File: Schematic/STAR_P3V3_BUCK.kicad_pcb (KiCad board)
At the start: 2 copper layers, 70.1 x 70 mm, 19 parts, among them J1 1017491, J2 6120XX21621_61200621621, J3 6120XX21621_61200821621, U1 TLV62569ADRLR

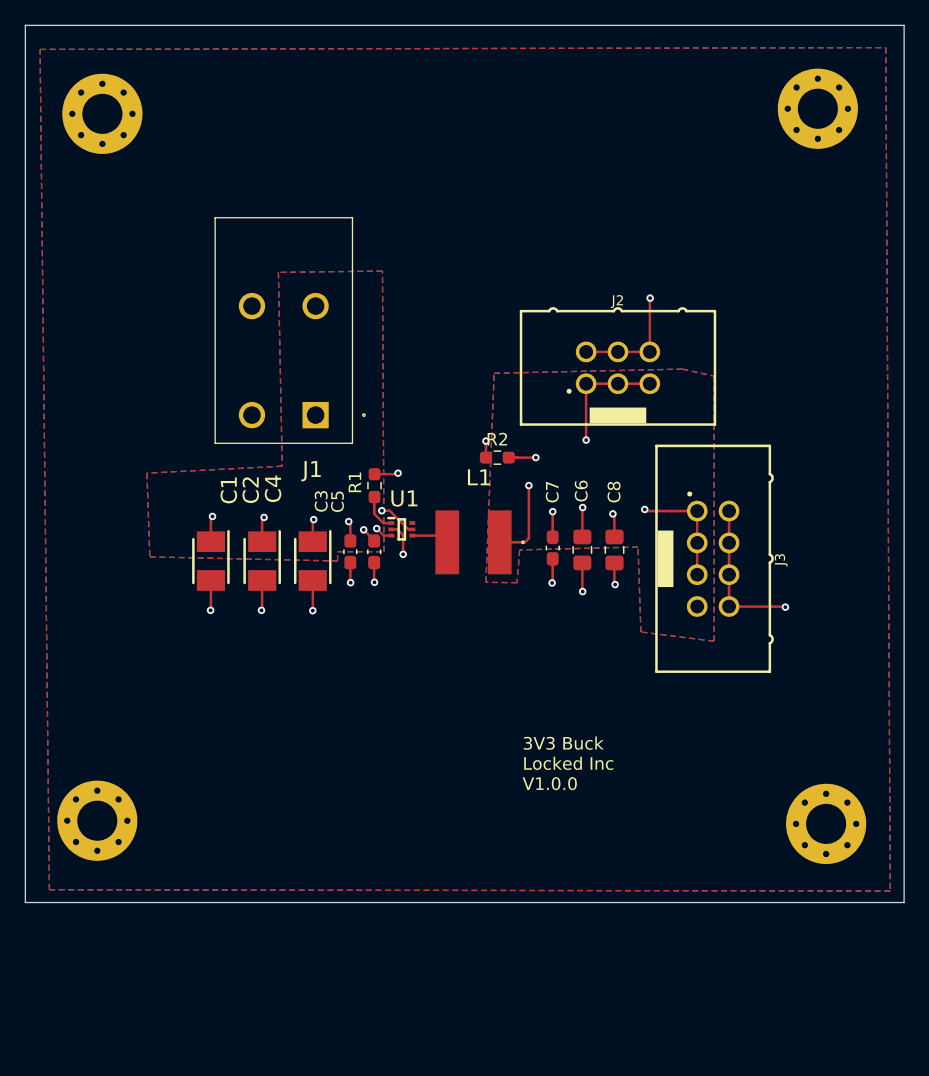
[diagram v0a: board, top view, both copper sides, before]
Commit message: V1.2.0
Lots Of changes, need help with screw holes
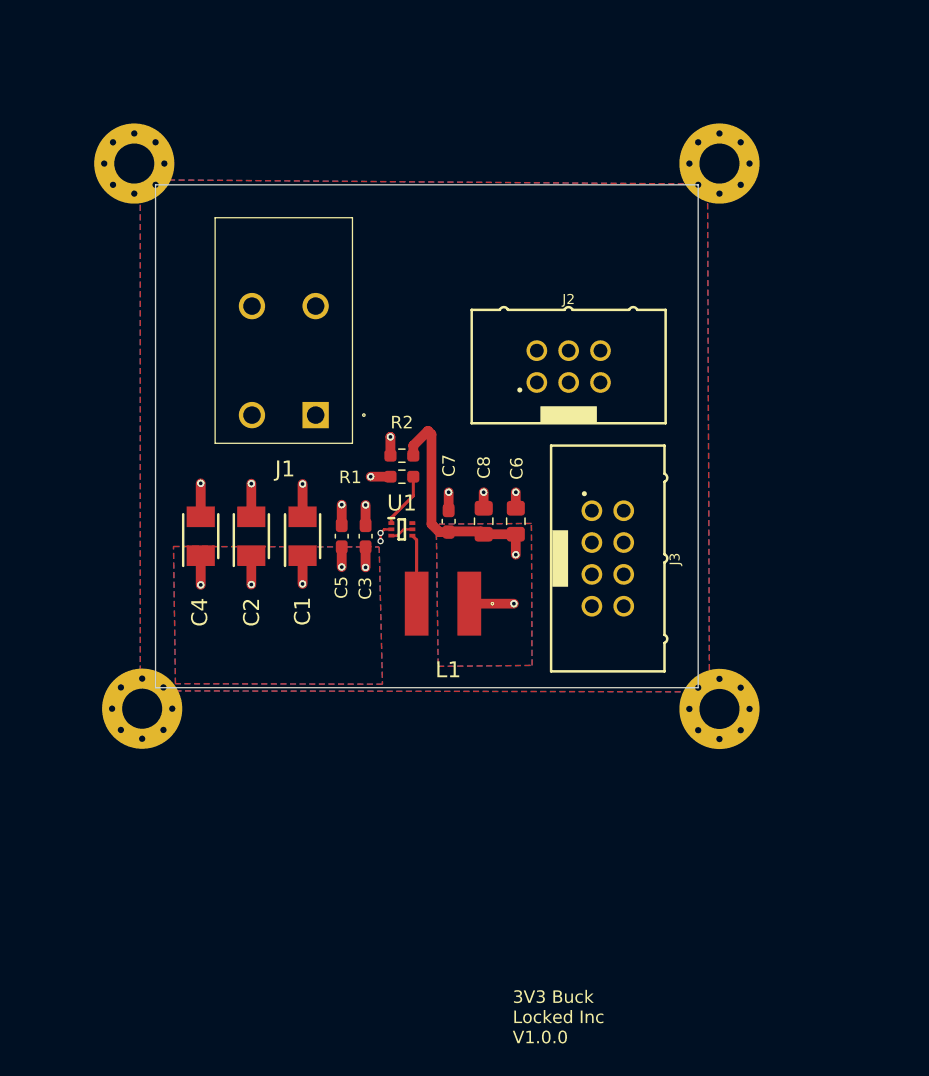
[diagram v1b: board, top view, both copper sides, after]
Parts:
- moved H4 12.5 mm to (190.0, 84.8)
- moved C8 10.7 mm to (171.2, 69.8), turned to -90 degrees
- moved H3 9.63 mm to (143.9, 84.8)
- moved C4 9.16 mm to (148.6, 71.0), turned to 90 degrees
- moved H2 8.99 mm to (190.0, 41.3)
- moved C7 8.58 mm to (168.4, 69.8), turned to 90 degrees
- moved J3 8.41 mm to (181.1, 72.8)
- moved R2 7.62 mm to (164.7, 64.6)
- moved C1 7.58 mm to (156.7, 71.0), turned to 90 degrees
- moved C6 5.78 mm to (173.8, 69.8), turned to 90 degrees
- moved L1 5.47 mm to (167.9, 76.4)
- moved H1 4.71 mm to (143.3, 41.3)
- moved J2 3.94 mm to (178.0, 57.5)
- moved C5 2.87 mm to (159.9, 71.0), turned to 90 degrees
- moved R1 2.30 mm to (164.7, 66.3), turned to 0 degrees
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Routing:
- net GND: track 43.8 -> 19.9 mm, vias 13 -> 12
- net /P3V3_BUCK: track 36.5 -> 22.4 mm, vias 7 -> 2
- net Net-(U1-SW): track 3.00 -> 5.57 mm
- net Net-(U1-FB): track 3.01 -> 4.44 mm
- net /P5V0_BUCK: track 13.1 -> 12.0 mm, vias 7 -> 5
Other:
- board size 70.1 x 70 mm -> 43.3 x 40.1 mm
